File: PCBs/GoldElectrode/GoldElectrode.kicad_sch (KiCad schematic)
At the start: 2 parts, among them J1 Finger, J2 Pad

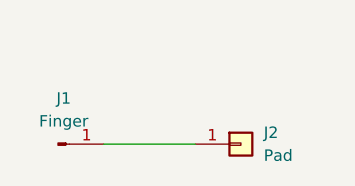
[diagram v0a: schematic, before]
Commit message: kicad changes
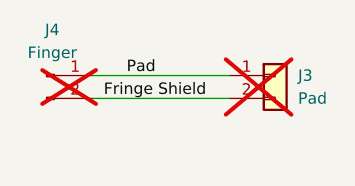
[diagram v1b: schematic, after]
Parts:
- removed J1: Finger, 4022S:Finger_01, symbol Connector:Conn_01x01_Pin
- removed J2: Pad, 4022S:Pad_20x20_mm, symbol Connector_Generic:Conn_01x01
- added J3: Pad, 4022S:Gold_electrode_pad, symbol Connector_Generic:Conn_01x02
- added J4: Finger, 4022S:Gold_electrode_finger, symbol Connector:Conn_01x02_Pin
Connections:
- new net Fringe Shield: J3.2 (Pin_2), J4.2 (Pin_2)
- new net Pad: J3.1 (Pin_1), J4.1 (Pin_1)
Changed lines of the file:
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@@
 	(wire
 		(pts
-			(xy 104.14 86.36) (xy 114.3 86.36)
+			(xy 102.87 81.28) (xy 118.11 81.28)
 		)
 		(stroke
@@
 		)
 	)
+	(wire
+		(pts
+			(xy 102.87 78.74) (xy 118.11 78.74)
+		)
+		(stroke
+			(width 0)
+			(type default)
+		)
+	)
+	(label "Fringe Shield"
+		(at 104.14 81.28 0)
+		(fields_autoplaced yes)
+		(effects
+			(font
+				(size 1.27 1.27)
+			)
+			(justify left bottom)
+		)
+	)
+	(label "Pad"
+		(at 106.68 78.74 0)
+		(fields_autoplaced yes)
+		(effects
+			(font
+				(size 1.27 1.27)
+			)
+			(justify left bottom)
+		)
+	)
 	(symbol
-		(lib_id "Connector:Conn_01x01_Pin")
-		(at 99.06 86.36 0)
+		(lib_id "Connector_Generic:Conn_01x02")
+		(at 123.19 78.74 0)
 		(unit 1)
 		(exclude_from_sim no)
 		(in_bom yes)
 		(on_board yes)
-		(dnp no)
+		(dnp yes)
 		(fields_autoplaced yes)
-		(property "Reference" "J1"
-			(at 99.695 81.28 0)
+		(property "Reference" "J3"
+			(at 125.73 78.7399 0)
 			(effects
 				(font
 					(size 1.27 1.27)
 				)
+				(justify left)
 			)
 		)
-		(property "Value" "Finger"
-			(at 99.695 83.82 0)
+		(property "Value" "Pad"
+			(at 125.73 81.2799 0)
 			(effects
 				(font
 					(size 1.27 1.27)
 				)
+				(justify left)
 			)
 		)
-		(property "Footprint" "4022S:Finger_01"
-			(at 99.06 86.36 0)
+		(property "Footprint" "4022S:Gold_electrode_pad"
+			(at 123.19 78.74 0)
 			(effects
 				(font
@@
 		)
 		(property "Datasheet" "~"
-			(at 99.06 86.36 0)
+			(at 123.19 78.74 0)
 			(effects
 				(font
@@
 			)
 		)
-		(property "Description" "Generic connector, single row, 01x01, script generated"
-			(at 99.06 86.36 0)
+		(property "Description" "Generic connector, single row, 01x02, script generated (kicad-library-utils/schlib/autogen/connector/)"
+			(at 123.19 78.74 0)
 			(effects
 				(font
@@
 		(pin "1"
 		)
+		(pin "2"
+		)
 		(instances
 			(project ""
 				(path "/47e5645b-2782-4f6e-807f-a2ecb5ce2a94"
-					(reference "J1")
+					(reference "J3")
 					(unit 1)
 				)
@@
 	)
 	(symbol
-		(lib_id "Connector_Generic:Conn_01x01")
-		(at 119.38 86.36 0)
+		(lib_id "Connector:Conn_01x02_Pin")
+		(at 97.79 78.74 0)
 		(unit 1)
 		(exclude_from_sim no)
 		(in_bom yes)
 		(on_board yes)
-		(dnp no)
+		(dnp yes)
 		(fields_autoplaced yes)
-		(property "Reference" "J2"
-			(at 121.92 85.0899 0)
+		(property "Reference" "J4"
+			(at 98.425 73.66 0)
 			(effects
 				(font
 					(size 1.27 1.27)
 				)
-				(justify left)
 			)
 		)
-		(property "Value" "Pad"
-			(at 121.92 87.6299 0)
+		(property "Value" "Finger"
+			(at 98.425 76.2 0)
 			(effects
 				(font
 					(size 1.27 1.27)
 				)
-				(justify left)
 			)
 		)
-		(property "Footprint" "4022S:Pad_20x20_mm"
-			(at 119.38 86.36 0)
+		(property "Footprint" "4022S:Gold_electrode_finger"
+			(at 97.79 78.74 0)
 			(effects
 				(font
@@
 		)
 		(property "Datasheet" "~"
-			(at 119.38 86.36 0)
+			(at 97.79 78.74 0)
 			(effects
 				(font
@@
 			)
 		)
-		(property "Description" "Generic connector, single row, 01x01, script generated (kicad-library-utils/schlib/autogen/connector/)"
-			(at 119.38 86.36 0)
+		(property "Description" "Generic connector, single row, 01x02, script generated"
+			(at 97.79 78.74 0)
 			(effects
 				(font
@@
 			)
 		)
+		(pin "2"
+		)
 		(pin "1"
 		)
@@
 			(project ""
 				(path "/47e5645b-2782-4f6e-807f-a2ecb5ce2a94"
-					(reference "J2")
+					(reference "J4")
 					(unit 1)
 				)
